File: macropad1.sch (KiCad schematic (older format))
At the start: 18 parts, among them J1 Conn_01x04, J2 USB_B_Mini, SW1 SW_Reed, SW2 Rotary_Encoder_Switch, U1 ATmega32U4-AU, Y1 16Mhz

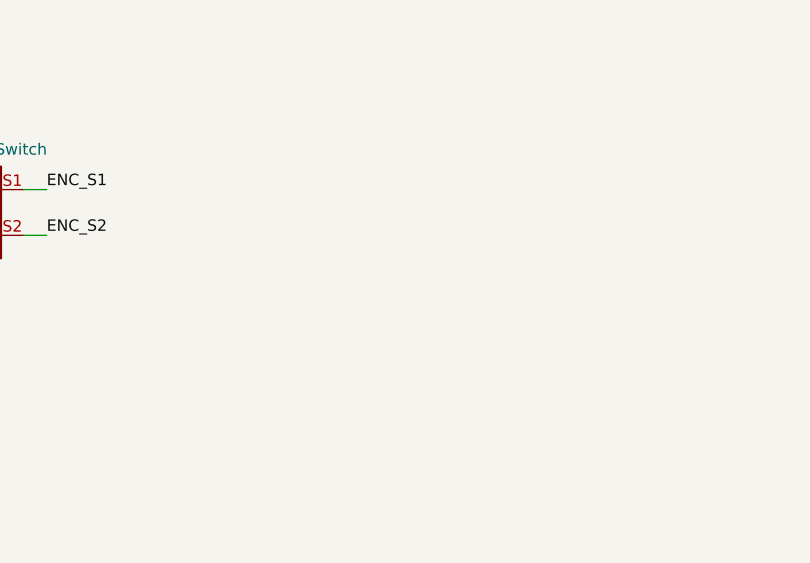
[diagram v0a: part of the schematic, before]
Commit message: Added artwork lib and eeprom
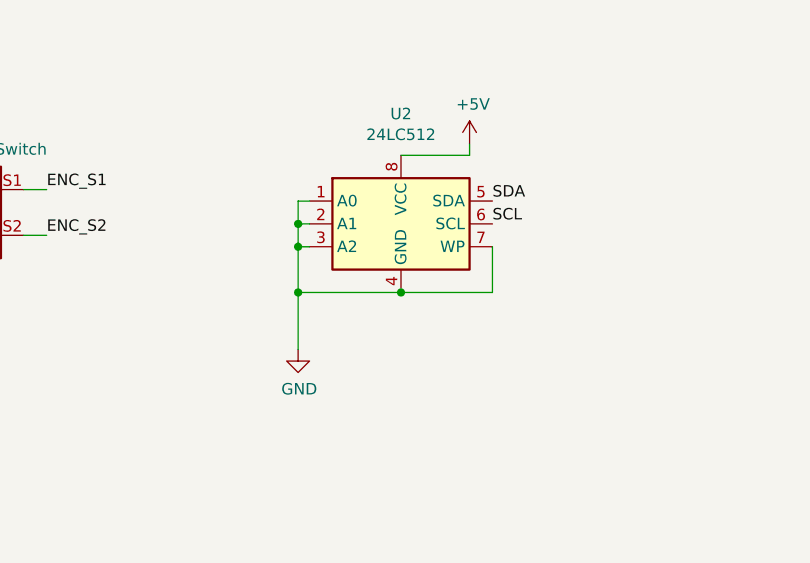
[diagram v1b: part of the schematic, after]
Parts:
- added U2: 24LC512, Package_SO:TSSOP-8_4.4x3mm_P0.65mm, symbol Memory_EEPROM:24LC512
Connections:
- net +5V: now also U2.8 (VCC)
- net GND: now also U2.1 (A0), U2.2 (A1), U2.3 (A2), U2.4 (GND), U2.7 (WP)
- net SCL: now also U2.6 (SCL)
- net SDA: now also U2.5 (SDA)
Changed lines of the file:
@@
 	1    0    0    -1
 $EndComp
+$Comp
+L Memory_EEPROM:24LC512 U2
+U 1 1 5F50FB6A
+P 7850 1600
+F 0 "U2" H 7850 2081 50  0000 C CNN
+F 1 "24LC512" H 7850 1990 50  0000 C CNN
+F 2 "Package_SO:TSSOP-8_4.4x3mm_P0.65mm" H 7850 1600 50  0001 C CNN
+F 3 "http://ww1.microchip.com/downloads/en/DeviceDoc/21754M.pdf" H 7850 1600 50  0001 C CNN
+	1    7850 1600
+	1    0    0    -1
+$EndComp
+Text Label 8250 1600 0    50   ~ 0
+SCL
+Text Label 8250 1500 0    50   ~ 0
+SDA
+Wire Wire Line
+	7450 1500 7400 1500
+Wire Wire Line
+	7400 1500 7400 1600
+$Comp
+L power:GND #PWR0115
+U 1 1 5F51AA52
+P 7400 2150
+F 0 "#PWR0115" H 7400 1900 50  0001 C CNN
+F 1 "GND" H 7405 1977 50  0000 C CNN
+F 2 "" H 7400 2150 50  0001 C CNN
+F 3 "" H 7400 2150 50  0001 C CNN
+	1    7400 2150
+	1    0    0    -1
+$EndComp
+Wire Wire Line
+	7450 1700 7400 1700
+Connection ~ 7400 1700
+Wire Wire Line
+	7450 1600 7400 1600
+Connection ~ 7400 1600
+Wire Wire Line
+	7400 1600 7400 1700
+Wire Wire Line
+	7400 1700 7400 1900
+Wire Wire Line
+	7850 1900 7400 1900
+Connection ~ 7400 1900
+Wire Wire Line
+	7400 1900 7400 2150
+$Comp
+L power:+5V #PWR0117
+U 1 1 5F52923E
+P 8150 1250
+F 0 "#PWR0117" H 8150 1100 50  0001 C CNN
+F 1 "+5V" H 8165 1423 50  0000 C CNN
+F 2 "" H 8150 1250 50  0001 C CNN
+F 3 "" H 8150 1250 50  0001 C CNN
+	1    8150 1250
+	1    0    0    -1
+$EndComp
+Wire Wire Line
+	7850 1300 8150 1300
+Wire Wire Line
+	8150 1300 8150 1250
+Wire Wire Line
+	8250 1700 8250 1900
+Wire Wire Line
+	8250 1900 7850 1900
+Connection ~ 7850 1900
 $EndSCHEMATC
